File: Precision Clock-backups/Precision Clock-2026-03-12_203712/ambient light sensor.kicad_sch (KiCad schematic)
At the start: 8 parts, among them Q3 DMN3008SFG

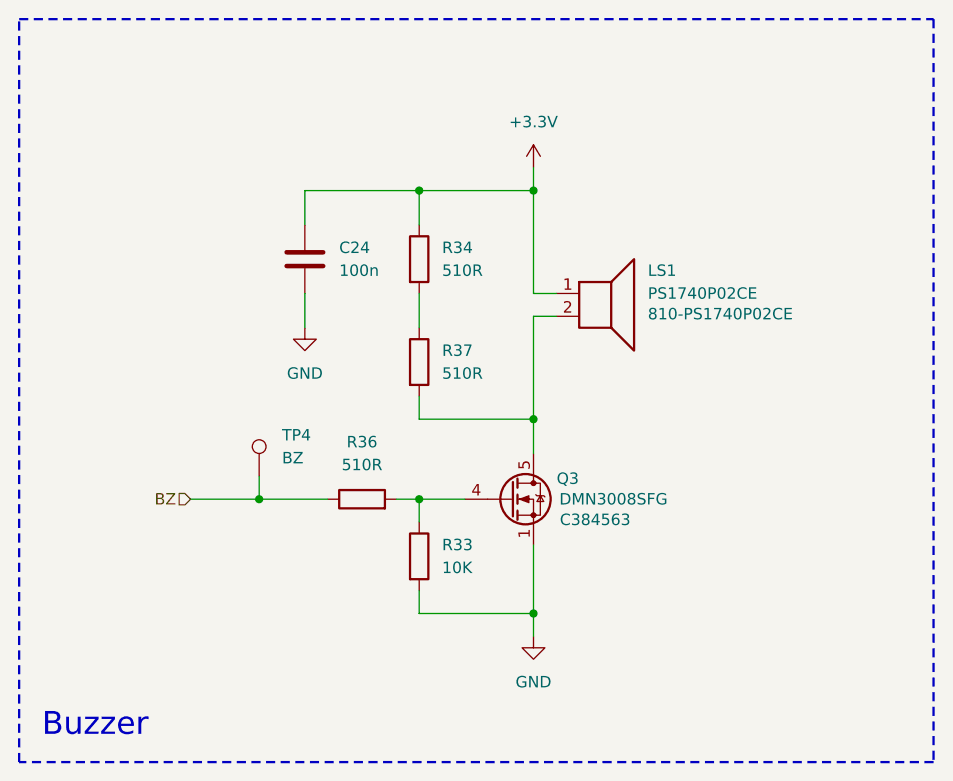
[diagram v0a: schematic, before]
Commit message: Routing
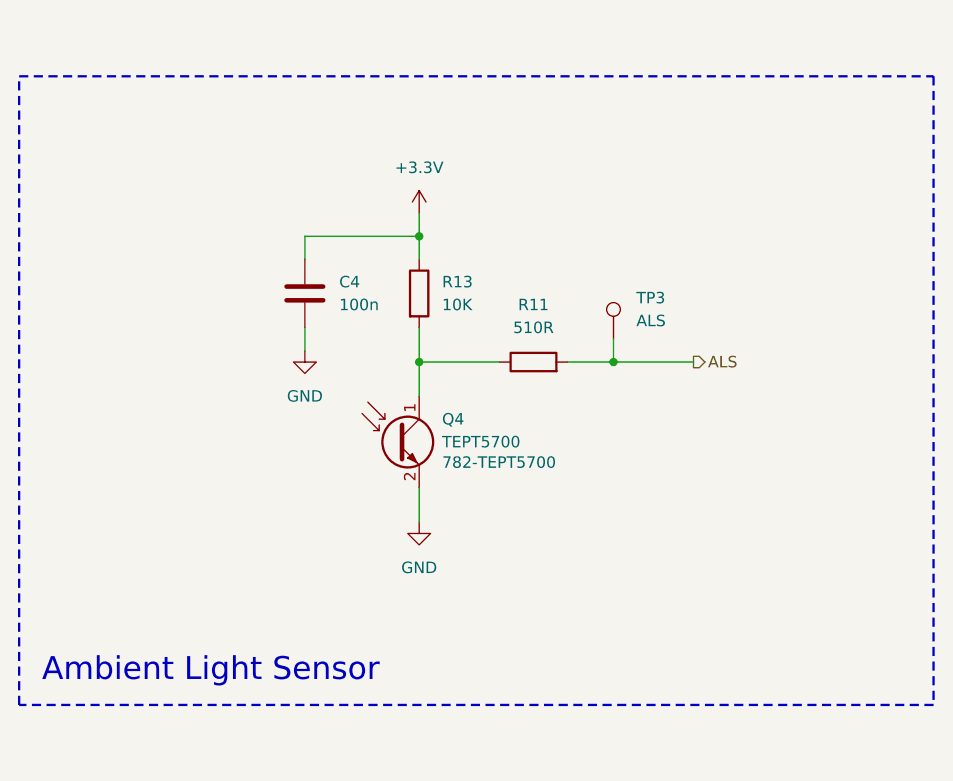
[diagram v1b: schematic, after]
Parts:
- removed C24: 100n, Capacitor_SMD:C_0402_1005Metric, symbol Device:C
- removed LS1: PS1740P02CE, precision_clock:TDK PS1740P02CE, symbol Device:Speaker
- removed Q3: DMN3008SFG, Package_SON:Diodes_PowerDI3333-8, symbol Transistor_FET:DMN3008SFG
- removed R33: 10K, Resistor_SMD:R_0402_1005Metric, symbol Device:R
- removed R34, R36, R37: 510R, Resistor_SMD:R_0402_1005Metric, symbol Device:R
- removed TP4: BZ, TestPoint:TestPoint_Pad_D1.0mm, symbol Connector:TestPoint
- added C4: 100n, Capacitor_SMD:C_0402_1005Metric, symbol Device:C
- added Q4: TEPT5700, LED_THT:LED_D5.0mm_Clear, symbol Sensor_Optical:TEPT4400
- added R11: 510R, Resistor_SMD:R_0402_1005Metric, symbol Device:R
- added R13: 10K, Resistor_SMD:R_0402_1005Metric, symbol Device:R
- added TP3: ALS, TestPoint:TestPoint_Pad_D1.0mm, symbol Connector:TestPoint
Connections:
- net +3.3V: now also C4.1, R13.1
- net GND: now also C4.2, Q4.2 (E)
- new net: Q4.1 (C), R11.1, R13.2
- new net ALS: R11.2, TP3.1
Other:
- note added: "Ambient Light Sensor"
- note removed: "Buzzer"
- title: Buzzer -> Ambient Light Sensor
